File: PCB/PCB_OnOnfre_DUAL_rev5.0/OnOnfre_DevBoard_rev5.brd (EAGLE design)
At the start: 44.1 x 44.2 mm, 30 parts, among them J3Y S8050, J7 8p, K1 OMRON-G3MB-202P-SSR2, K2 OMRON-G3MB-202P-SSR2, U2 esp12

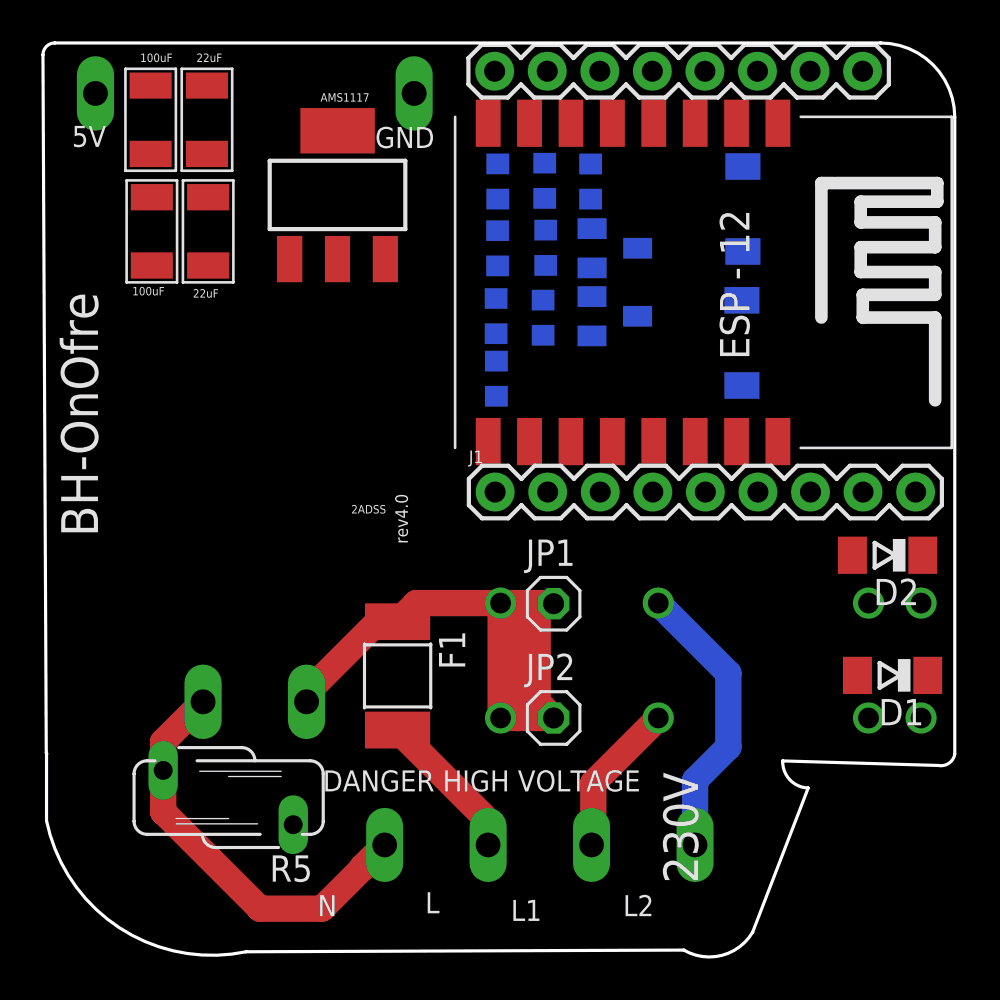
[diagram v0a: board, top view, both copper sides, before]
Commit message: rev5
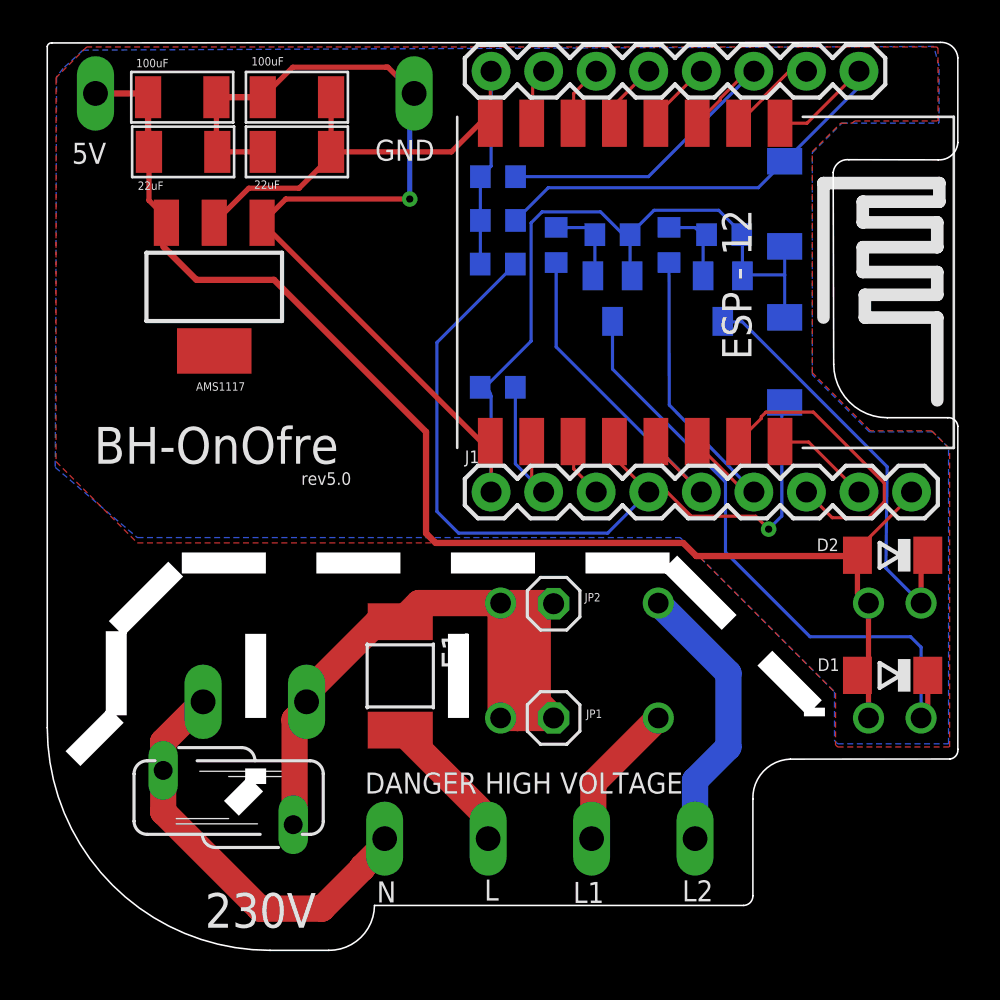
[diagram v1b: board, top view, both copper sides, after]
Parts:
- moved C4 9.55 mm to (12.8, 43.7), turned to 180 degrees
- moved R2 8.65 mm to (33.4, 37.1), turned to 0 degrees
- moved AMS1117 7.43 mm to (8.77, 34.6), turned to 180 degrees
- moved R1 7.02 mm to (30.7, 36.6)
- moved C1 5.76 mm to (12.8, 41.1), turned to 180 degrees
- moved JY3 5.75 mm to (33.3, 34.0), turned to 180 degrees
- moved R3 5.58 mm to (28.0, 37.1), turned to 0 degrees
- moved R10 4.85 mm to (22.5, 37.8), turned to 0 degrees
- moved R8 4.62 mm to (22.5, 35.7), turned to 0 degrees
- moved R4 4.50 mm to (25.3, 36.6)
- moved FLASH 2.22 mm to (36.3, 31.0)
- moved RESET 2.03 mm to (36.3, 38.6)
- moved C2 1.93 mm to (7.26, 41.1), turned to 0 degrees
- moved C3 1.88 mm to (7.22, 43.7), turned to 0 degrees
- moved J3Y 0.86 mm to (28.0, 34.0), turned to 180 degrees
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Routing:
- net GND: track 0.00 -> 87.2 mm, vias 0 -> 1
- net VCC: track 0.00 -> 68.2 mm
- net GPIO0: track 0.00 -> 41.2 mm, vias 0 -> 1
- net 3V3: track 0.00 -> 31.5 mm
- net N$1: track 0.00 -> 30.4 mm
- net RESET: track 0.00 -> 24.9 mm
- net N$9: track 0.00 -> 20.6 mm
- net CH_PD: track 0.00 -> 17.5 mm
- net GPIO04: track 0.00 -> 17.4 mm
- net GPIO05: track 0.00 -> 16.6 mm
- net RX: track 0.00 -> 14.6 mm
- net GPIO15: track 0.00 -> 8.31 mm
- net LINE_L: track 33.9 -> 40.0 mm
- net TX: track 0.00 -> 4.83 mm
- net ADC: track 0.00 -> 4.36 mm
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- added copper zone on layer 1, net GND
- added copper zone on layer 16, net GND
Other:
- board size 44.1 x 44.2 mm -> 44 x 43.9 mm
- board text added: "rev5.0"
- board text removed: "2ADSS"
- board text removed: "rev4.0"

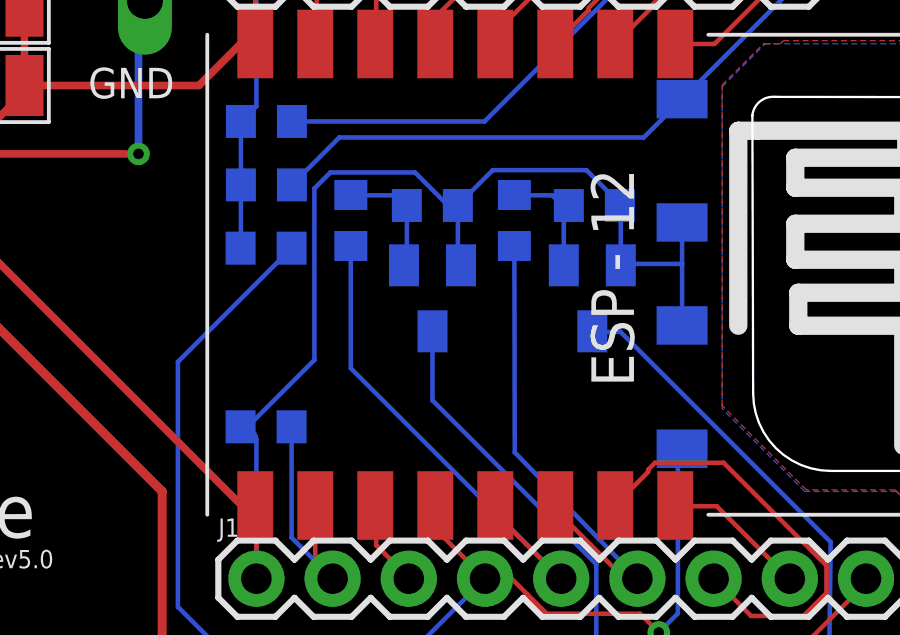
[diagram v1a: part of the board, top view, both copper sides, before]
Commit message: rev 5
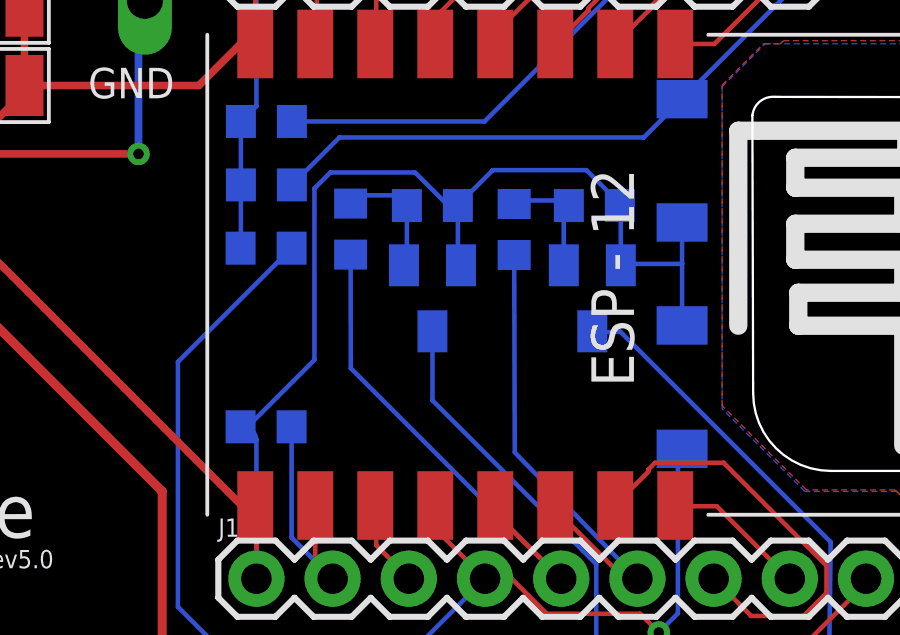
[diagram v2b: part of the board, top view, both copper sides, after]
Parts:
- moved R1 0.30 mm to (30.7, 36.3)
- moved R4 0.29 mm to (25.3, 36.3)
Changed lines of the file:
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@@
 <attribute name="NAME" x="27.612609375" y="31.9995125" size="0.4064" layer="26" rot="MR180"/>
 </element>
-<element name="R4" library="resistor" library_urn="urn:adsk.eagle:library:348" package="R0603" package3d_urn="urn:adsk.eagle:package:26057/1" value="10k" x="25.291903125" y="36.57466875" smashed="yes" rot="MR90">
-<attribute name="VALUE" x="25.05305625" y="34.841740625" size="0.4064" layer="26" rot="MR180"/>
+<element name="R4" library="resistor" library_urn="urn:adsk.eagle:library:348" package="R0603" package3d_urn="urn:adsk.eagle:package:26057/1" value="10k" x="25.285528125" y="36.287934375" smashed="yes" rot="MR90">
+<attribute name="VALUE" x="25.04668125" y="34.55500625" size="0.4064" layer="26" rot="MR180"/>
 </element>
 <element name="C4" library="Seeed-Capacitor" library_urn="urn:adsk.eagle:library:464" package="C1206" package3d_urn="urn:adsk.eagle:package:32384/1" value="100uF" x="12.762778125" y="43.71605" smashed="yes" rot="R180">
@@
 </element>
 <element name="JY3" library="semicon-smd-ipc" library_urn="urn:adsk.eagle:library:353" package="SOT23" package3d_urn="urn:adsk.eagle:package:26310/1" value="S8050 " x="33.341853125" y="33.98164375" smashed="yes" rot="MR180"/>
-<element name="R1" library="resistor" library_urn="urn:adsk.eagle:library:348" package="R0603" package3d_urn="urn:adsk.eagle:package:26057/1" value="10k" x="30.744346875" y="36.57466875" smashed="yes" rot="MR90">
-<attribute name="VALUE" x="30.28205" y="34.8799875" size="0.4064" layer="26" rot="MR180"/>
+<element name="R1" library="resistor" library_urn="urn:adsk.eagle:library:348" package="R0603" package3d_urn="urn:adsk.eagle:package:26057/1" value="10k" x="30.737975" y="36.27514375" smashed="yes" rot="MR90">
+<attribute name="VALUE" x="30.275678125" y="34.5804625" size="0.4064" layer="26" rot="MR180"/>
 </element>
 <element name="J7" library="SparkFun-Connectors" library_urn="urn:adsk.eagle:library:513" package="1X08" package3d_urn="urn:adsk.eagle:package:38138/1" value="8p" x="22.145709375" y="44.971115625" smashed="yes">
@@
 <wire x1="32.560315625" y1="37.0737625" x2="32.391853125" y2="36.966671875" width="0.1524" layer="16"/>
 <wire x1="32.391853125" y1="36.966671875" x2="32.391853125" y2="35.08164375" width="0.1524" layer="16"/>
-<wire x1="32.004" y1="37.4142" x2="30.7848" y2="37.4142" width="0.1524" layer="16"/>
-<wire x1="32.385" y1="37.0332" x2="32.004" y2="37.4142" width="0.1524" layer="16"/>
-<wire x1="30.7848" y1="37.4142" x2="30.744346875" y2="37.42466875" width="0.1524" layer="16"/>
+<wire x1="32.341725" y1="37.24213125" x2="31.122525" y2="37.24213125" width="0.1524" layer="16"/>
+<wire x1="32.385" y1="37.0332" x2="32.341725" y2="37.24213125" width="0.1524" layer="16"/>
+<wire x1="31.122525" y1="37.24213125" x2="30.737975" y2="37.12514375" width="0.1524" layer="16"/>
 <wire x1="32.385" y1="37.0332" x2="32.560315625" y2="37.0737625" width="0.1524" layer="16"/>
 </signal>
@@
 <wire x1="26.8224" y1="37.4142" x2="25.2984" y2="37.4142" width="0.1524" layer="16"/>
 <wire x1="27.1272" y1="37.1094" x2="26.8224" y2="37.4142" width="0.1524" layer="16"/>
-<wire x1="25.2984" y1="37.4142" x2="25.291903125" y2="37.42466875" width="0.1524" layer="16"/>
+<wire x1="25.2984" y1="37.4142" x2="25.285528125" y2="37.137934375" width="0.1524" layer="16"/>
 <wire x1="27.1272" y1="37.1094" x2="27.160934375" y2="37.0737625" width="0.1524" layer="16"/>
 </signal>
@@
 <contactref element="J1" pad="5"/>
 <contactref element="R4" pad="1"/>
-<wire x1="25.291903125" y1="35.72466875" x2="25.291903125" y2="31.648796875" width="0.1524" layer="16"/>
+<wire x1="25.285528125" y1="35.437934375" x2="25.291903125" y2="31.648796875" width="0.1524" layer="16"/>
 <wire x1="25.291903125" y1="31.648796875" x2="32.305709375" y2="24.634990625" width="0.1524" layer="16"/>
 <wire x1="30.1752" y1="26.7462" x2="30.1752" y2="27.051" width="0.1524" layer="1"/>
@@
 <contactref element="J1" pad="6"/>
 <contactref element="R1" pad="1"/>
-<wire x1="30.744346875" y1="35.72466875" x2="30.757090625" y2="28.844690625" width="0.1524" layer="16"/>
+<wire x1="30.737975" y1="35.42514375" x2="30.757090625" y2="28.844690625" width="0.1524" layer="16"/>
 <wire x1="30.757090625" y1="28.844690625" x2="34.845709375" y2="24.634990625" width="0.1524" layer="16"/>
 <wire x1="32.1564" y1="26.8986" x2="32.1564" y2="27.051" width="0.1524" layer="1"/>
